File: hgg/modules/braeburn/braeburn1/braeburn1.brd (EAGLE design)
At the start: 100 x 70.5 mm, 50 parts, among them IC1 MAX481CSA, IC2 MEGA8-AI, IC3 LM324D, IC4 LM2574N-12, IC5 LM2574N-5.0, IC6 LM2574N-3.3, Q1 20MHz

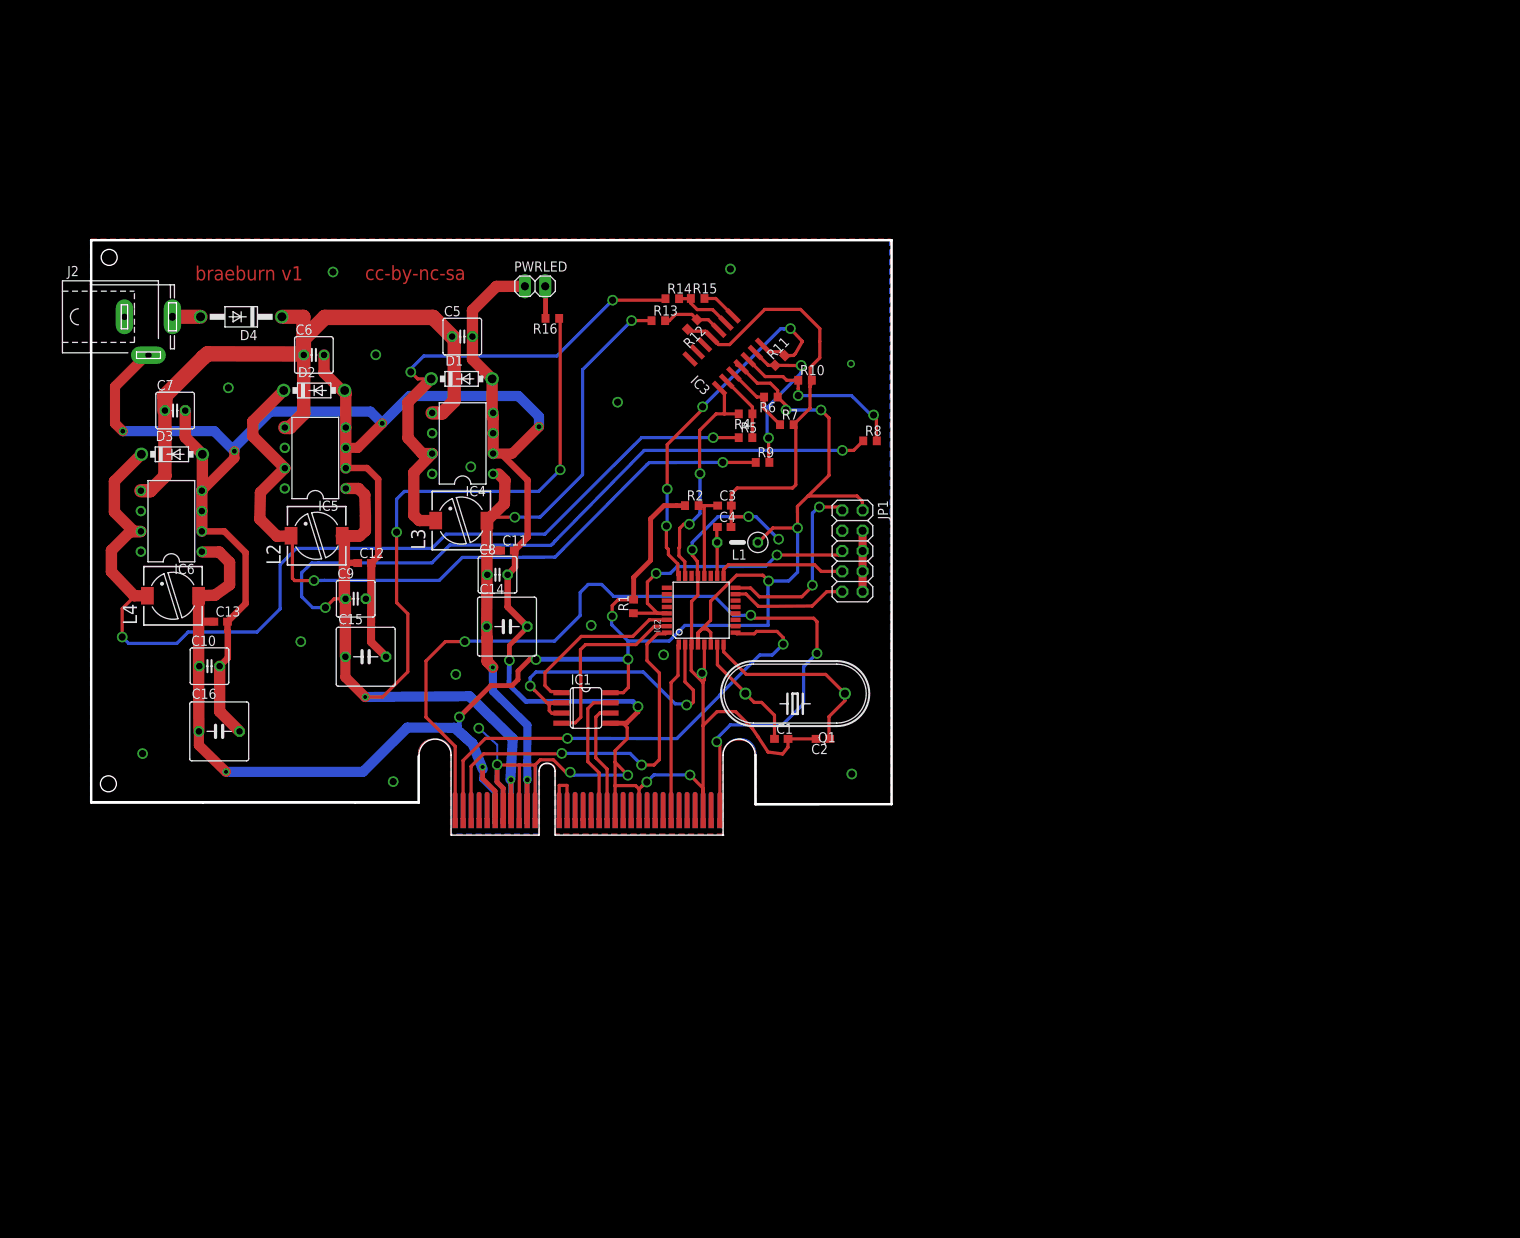
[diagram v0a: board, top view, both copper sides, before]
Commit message: new release of braeburn board file
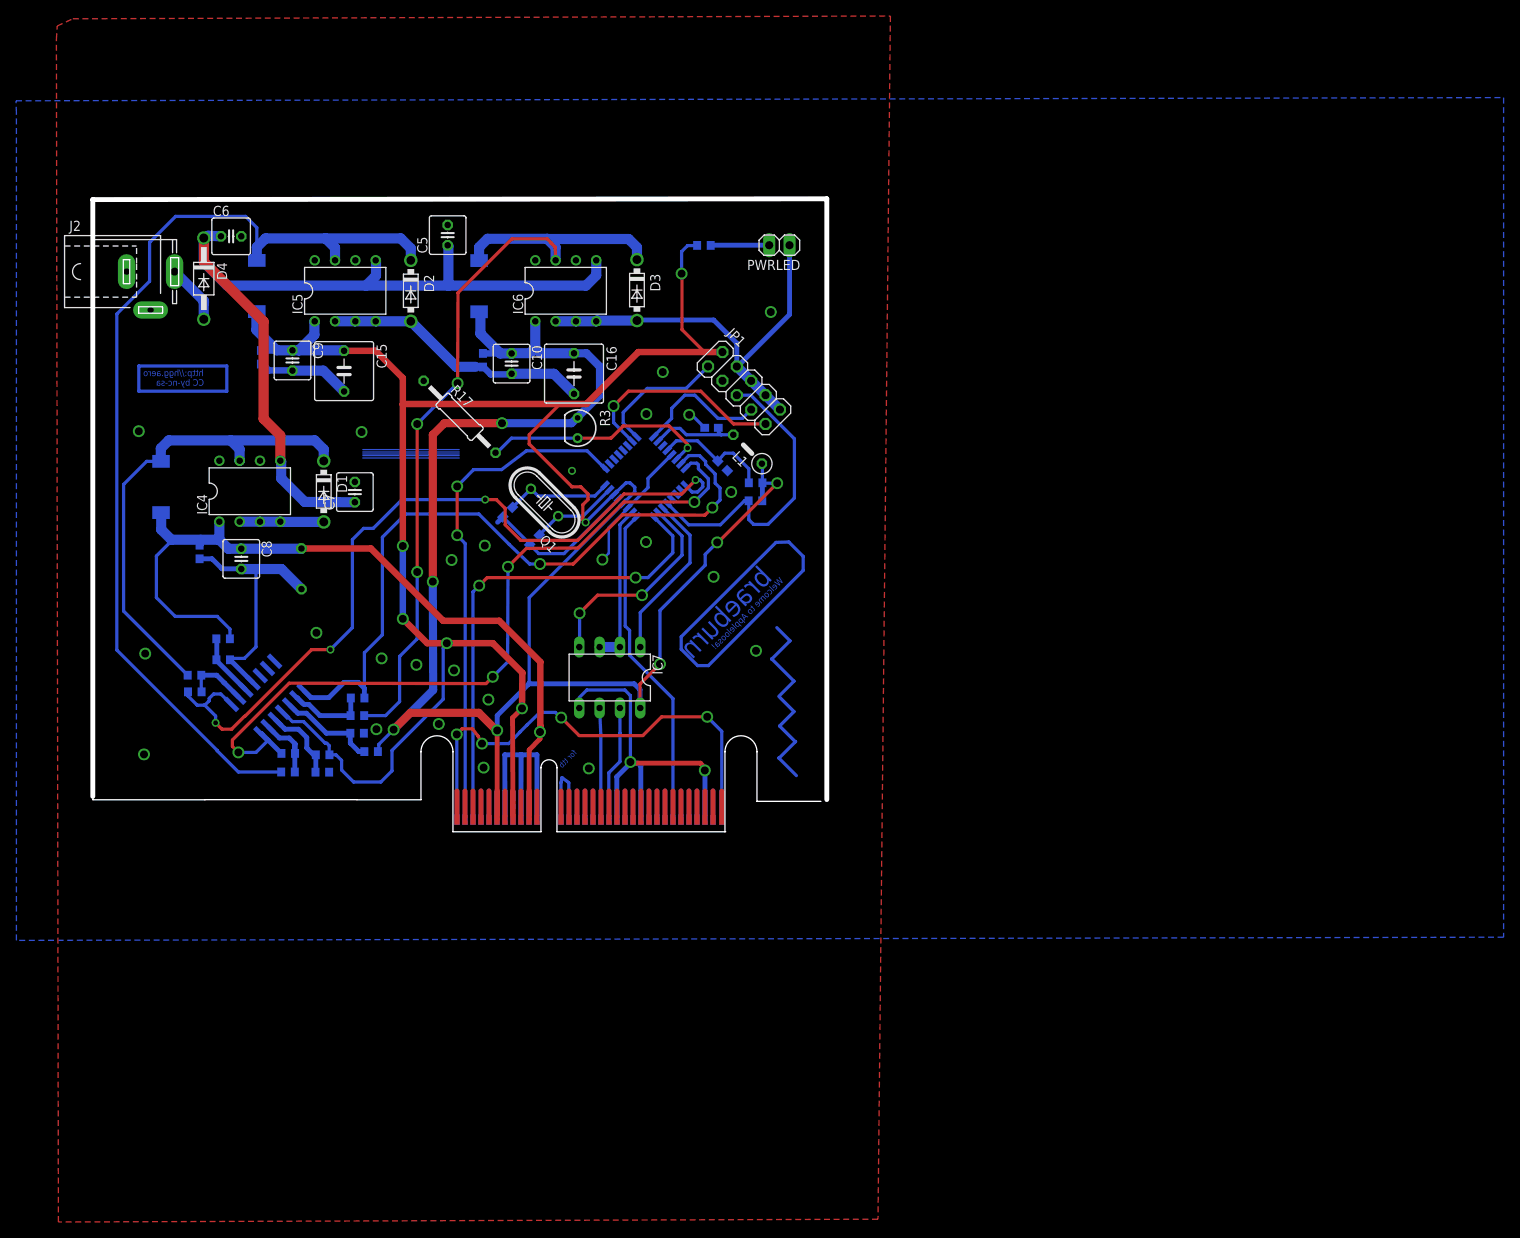
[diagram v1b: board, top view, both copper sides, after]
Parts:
- removed IC1: MAX481CSA, maxim:SO08
- added IC7: LTC485N, linear-technology:DIL08
- added R17: 1k, rcl:0207/12
- added R3: PTC-SOD70, ptc-ntc:SOD70
- Q1: value 20MHz -> 8-20MHz; device crystal:HC33U-V -> crystal:HC49/S
- R1: value (none) -> 10k
- moved R15 79.8 mm to (12.9, 17.9), flipped to the bottom
- moved R8 78.9 mm to (28.9, 10.0), flipped to the bottom
- moved R11 78.7 mm to (24.6, 10.2), flipped to the bottom, turned to 0 degrees
- moved R10 77.7 mm to (28.8, 7.83), flipped to the bottom, turned to 180 degrees
- moved R14 76.0 mm to (12.9, 19.9), flipped to the bottom, turned to 180 degrees
- moved R12 72.1 mm to (16.4, 21.9), flipped to the bottom, turned to 180 degrees
- moved IC3 71.8 mm to (22.0, 17.2), flipped to the bottom, turned to 315 degrees
- moved R9 70.8 mm to (24.6, 7.85), flipped to the bottom, turned to 180 degrees
- moved R13 67.4 mm to (16.4, 24.5), flipped to the bottom
- moved R6 66.8 mm to (34.9, 10.4), flipped to the bottom, turned to 0 degrees
- moved R7 66.1 mm to (33.2, 12.7), flipped to the bottom, turned to 180 degrees
- moved C16 63.0 mm to (60.3, 57.6), turned to 270 degrees
- moved D3 61.7 mm to (68.2, 68.1), turned to 270 degrees
- moved R4 60.1 mm to (33.2, 17.1), flipped to the bottom
- moved R5 59.7 mm to (33.2, 14.9), flipped to the bottom
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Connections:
- removed net M_12V: IC3.8, R15.2
- new net PTC: IC2.22, R17.2, R3.2
- net BUS0+: now also IC7.7; no longer IC1.6
- net BUS0-: now also IC7.6; no longer IC1.7
- net GND: now also IC7.5, R17.1; no longer IC1.5, U$1.B07(GND), U$1.B11(GND)
- net M12V: now also IC3.8, R15.2
- net N$4: now also Q1.1; no longer Q1.2
- net N$5: now also Q1.2; no longer Q1.1
- net OUT_12V: no longer U$1.A10(+12V)
- net OUT_3V3: now also IC7.8, R3.1; no longer IC1.8, IC2.4, IC2.6, IC3.4, JP1.2, U$1.A06(+3V3)
- net OUT_5V: now also IC2.4, IC2.6, IC3.4, JP1.2; no longer U$1.A08(+5V)
- net RW: now also IC7.2, IC7.3; no longer IC1.2, IC1.3
- net RX: now also IC7.1; no longer IC1.1
- net TX: now also IC7.4; no longer IC1.4
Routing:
- net GND: track 515.2 -> 264.6 mm, vias 29 -> 27
- net M12V: track 0.00 -> 100.0 mm, vias 0 -> 4
- net M3V3: track 29.2 -> 88.8 mm
- net N$1: track 112.6 -> 60.7 mm
- net M5V: track 47.5 -> 95.1 mm
- net N$6: track 0.00 -> 45.2 mm
- net N_3V3: track 145.7 -> 103.3 mm, vias 2 -> 3
- net OUT_3V3: track 249.7 -> 215.9 mm, vias 10 -> 7
- net N_5V: track 94.9 -> 125.6 mm, vias 2 -> 0
- net PTC: track 0.00 -> 28.6 mm, vias 0 -> 1
- net N$3: track 0.00 -> 28.3 mm, vias 1 -> 0
- net RW: track 40.0 -> 20.0 mm, vias 2 -> 0
- net PPS: track 22.7 -> 40.9 mm
- net DCIN: track 95.3 -> 111.2 mm
- net N$9: track 0.00 -> 14.0 mm
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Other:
- board size 100 x 70.5 mm -> 91.8 x 75.1 mm
- board text added: "CC by-nc-sa"
- board text added: "Welcome to Appleloosa!"
- board text added: "braeburn"
- board text added: "for ttb"
- board text added: "http://hgg.aero"
- board text removed: "braeburn v1"
- board text removed: "cc-by-nc-sa"
